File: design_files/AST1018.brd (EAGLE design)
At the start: 10 x 11 mm, 7 parts, among them J1 SM05B, J2 SM05B, J3 BM05B, J4 BM05B, U1 SK6812MINI

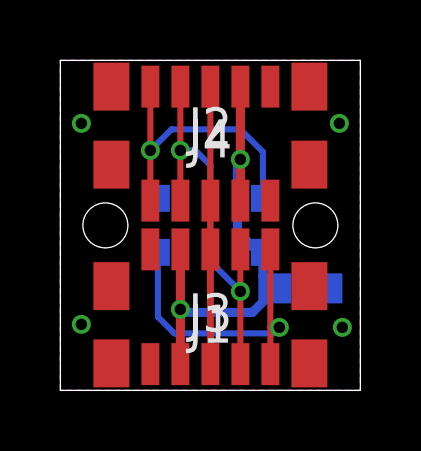
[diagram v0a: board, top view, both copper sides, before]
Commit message: updated documentation
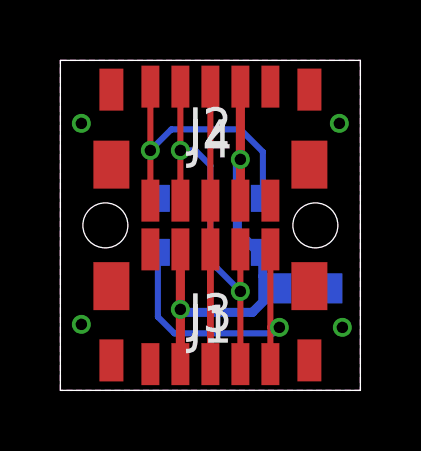
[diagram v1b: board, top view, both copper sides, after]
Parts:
- J1, J2: device tinycircuits:JST_SH_5X1 -> tinycircuits:JST_SH_5X1_EDGE
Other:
- board text added: "Wireling RGB LED"
- board text removed: "Serial RGB LED - Double Con."
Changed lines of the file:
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@@
 <layer number="54" name="bGND_GNDA" color="7" fill="1" visible="yes" active="yes"/>
 <layer number="56" name="wert" color="7" fill="1" visible="yes" active="yes"/>
+<layer number="57" name="tCAD" color="7" fill="1" visible="no" active="no"/>
+<layer number="58" name="bCAD" color="7" fill="1" visible="no" active="no"/>
+<layer number="59" name="Invisible" color="7" fill="1" visible="no" active="no"/>
+<layer number="61" name="stand" color="7" fill="1" visible="no" active="no"/>
+<layer number="88" name="SimResults" color="9" fill="1" visible="yes" active="yes"/>
+<layer number="89" name="SimProbes" color="9" fill="1" visible="yes" active="yes"/>
+<layer number="90" name="Modules" color="5" fill="1" visible="yes" active="yes"/>
 <layer number="91" name="Nets" color="2" fill="1" visible="no" active="no"/>
 <layer number="92" name="Busses" color="1" fill="1" visible="no" active="no"/>
@@
 <layer number="97" name="Info" color="7" fill="1" visible="no" active="no"/>
 <layer number="98" name="Guide" color="6" fill="1" visible="no" active="no"/>
+<layer number="99" name="SpiceOrder" color="5" fill="1" visible="no" active="no"/>
 <layer number="100" name="Muster" color="7" fill="1" visible="yes" active="yes"/>
 <layer number="101" name="Patch_Top" color="7" fill="1" visible="yes" active="yes"/>
@@
 <layer number="111" name="tGTest" color="4" fill="1" visible="no" active="no"/>
 <layer number="112" name="bGTest" color="1" fill="1" visible="no" active="no"/>
+<layer number="113" name="HENWAY_PKG" color="12" fill="1" visible="yes" active="yes"/>
+<layer number="114" name="50_Electronics_Plate" color="7" fill="1" visible="yes" active="yes"/>
+<layer number="115" name="henwayRES" color="5" fill="1" visible="yes" active="yes"/>
 <layer number="116" name="Patch_BOT" color="7" fill="1" visible="yes" active="yes"/>
 <layer number="117" name="mPads" color="7" fill="1" visible="no" active="no"/>
@@
 <layer number="151" name="HeatSink" color="7" fill="1" visible="yes" active="yes"/>
 <layer number="152" name="mbDocu" color="7" fill="1" visible="no" active="no"/>
+<layer number="153" name="FabDoc1" color="6" fill="1" visible="no" active="no"/>
+<layer number="154" name="FabDoc2" color="2" fill="1" visible="no" active="no"/>
+<layer number="155" name="FabDoc3" color="7" fill="15" visible="no" active="no"/>
+<layer number="156" name="bCapacitor" color="7" fill="1" visible="yes" active="yes"/>
+<layer number="157" name="tResistor" color="7" fill="1" visible="yes" active="yes"/>
+<layer number="158" name="bResistor" color="7" fill="1" visible="yes" active="yes"/>
+<layer number="159" name="henwayCAP" color="13" fill="1" visible="yes" active="yes"/>
+<layer number="160" name="IDFDebug" color="7" fill="1" visible="yes" active="yes"/>
 <layer number="191" name="mNets" color="7" fill="1" visible="no" active="no"/>
 <layer number="192" name="mBusses" color="7" fill="1" visible="no" active="no"/>
@@
 <layer number="223" name="223bmp" color="7" fill="1" visible="yes" active="yes"/>
 <layer number="224" name="224bmp" color="7" fill="1" visible="yes" active="yes"/>
+<layer number="231" name="Eagle3D_PG1" color="7" fill="1" visible="yes" active="yes"/>
+<layer number="232" name="Eagle3D_PG2" color="7" fill="1" visible="yes" active="yes"/>
+<layer number="233" name="Eagle3D_PG3" color="7" fill="1" visible="yes" active="yes"/>
 <layer number="248" name="Housing" color="7" fill="1" visible="yes" active="yes"/>
 <layer number="249" name="Edge" color="7" fill="1" visible="yes" active="yes"/>
@@
 <wire x1="0" y1="40.8" x2="0" y2="0" width="0.127" layer="48"/>
 <dimension x1="15" y1="21" x2="25" y2="21" x3="20" y3="22.454653125" layer="48"/>
-<text x="38.111025" y="4.365003125" size="0.889" layer="48">Serial RGB LED - Double Con.</text>
+<text x="38.111025" y="4.365003125" size="0.889" layer="48">Wireling RGB LED</text>
 <text x="34.986825" y="1.7714" size="0.889" layer="48">AS-PCB-AST1018</text>
 <text x="57.3810375" y="1.6952" size="0.889" layer="48">2</text>
@@
 <attribute name="NO_BOM" value="TRUE" x="34" y="0" size="1.778" layer="27" display="off"/>
 </element>
-<element name="J1" library="tinycircuits" package="JST_SH_5X1" value="SM05B" x="20" y="12.225">
+<element name="J1" library="tinycircuits" package="JST_SH_5X1_EDGE" value="SM05B" x="20" y="12.225">
 <attribute name="PARTNO" value="AS-ITM-00340" x="20" y="12.225" size="1.778" layer="27" display="off"/>
 <attribute name="VALUE" value="SM05B" x="20" y="12.225" size="1.778" layer="27" display="off"/>
@@
 <attribute name="VALUE" value="SK6812MINI" x="20" y="15.5" size="1.778" layer="28" rot="MR180" display="off"/>
 </element>
-<element name="J2" library="tinycircuits" package="JST_SH_5X1" value="SM05B" x="20" y="18.8" rot="R180">
+<element name="J2" library="tinycircuits" package="JST_SH_5X1_EDGE" value="SM05B" x="20" y="18.8" rot="R180">
 <attribute name="PARTNO" value="AS-ITM-00340" x="20" y="18.8" size="1.778" layer="27" rot="R180" display="off"/>
 <attribute name="PNPROTATION" value="180" x="20" y="18.8" size="1.778" layer="27" rot="R180" display="off"/>
@@
 <attribute name="PARTNO" value="AS-ITM-00391" x="20" y="12.6" size="1.778" layer="27" display="off"/>
 <attribute name="VALUE" value="BM05B" x="20" y="12.6" size="1.778" layer="27" display="off"/>
+<attribute name="PNPROTATION" value="0" x="20" y="12.6" size="1.778" layer="27" display="off"/>
 </element>
 <element name="J4" library="tinycircuits" package="JST_SH_5X1_VERT" value="BM05B" x="20" y="18.4" rot="R180">
@@
 <attribute name="VALUE" value="BM05B" x="20" y="18.4" size="1.778" layer="27" rot="R180" display="off"/>
 <attribute name="DATABASE" value="./../../../../../Components/TinyCircuits_Part_Database.txt" x="20" y="18.4" size="1.778" layer="27" rot="R180" display="off"/>
+<attribute name="PNPROTATION" value="0" x="20" y="18.4" size="1.778" layer="27" rot="R180" display="off"/>
 </element>
 <element name="C1" library="tinycircuits" package="C0603" value="1uF" x="23" y="13.4" rot="MR180">
@@
 </signal>
 </signals>
-<errors>
-</errors>
 </board>
 </drawing>
